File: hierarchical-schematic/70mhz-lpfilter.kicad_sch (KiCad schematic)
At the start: 11 parts, among them J701 In, J702 Out

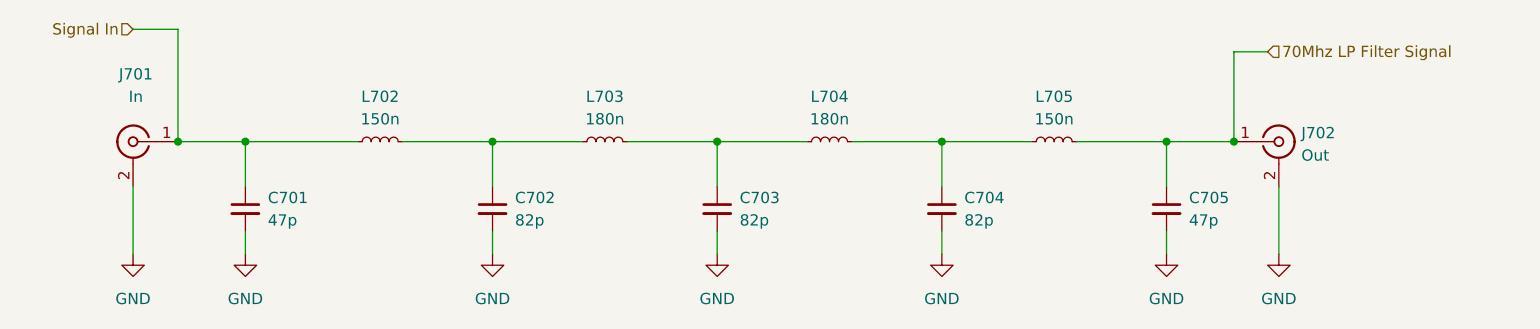
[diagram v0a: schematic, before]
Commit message: v7 conversion
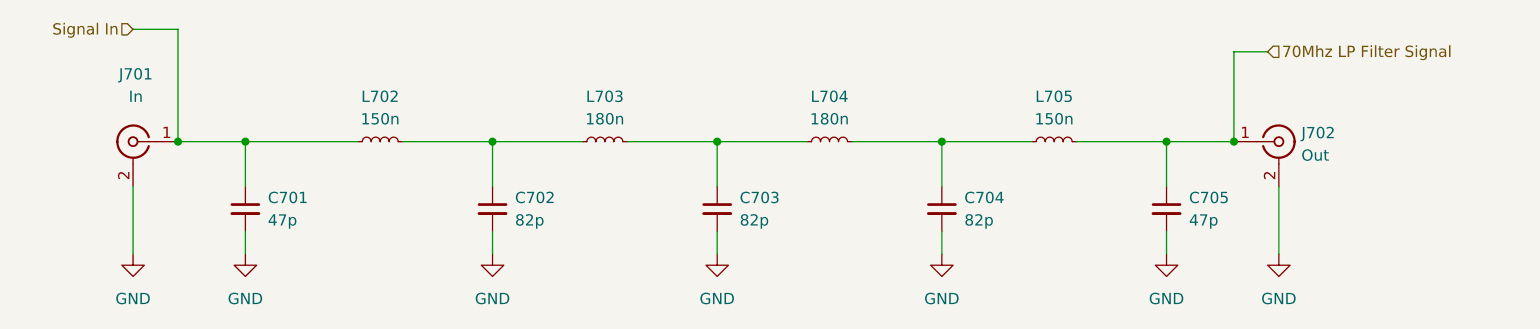
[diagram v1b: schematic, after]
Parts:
- J701, J702: Spice_Model Conn_Coaxial -> (none); Spice_Netlist_Enabled N -> (none); Spice_Primitive J -> (none)
